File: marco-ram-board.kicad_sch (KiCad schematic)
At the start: 0 parts

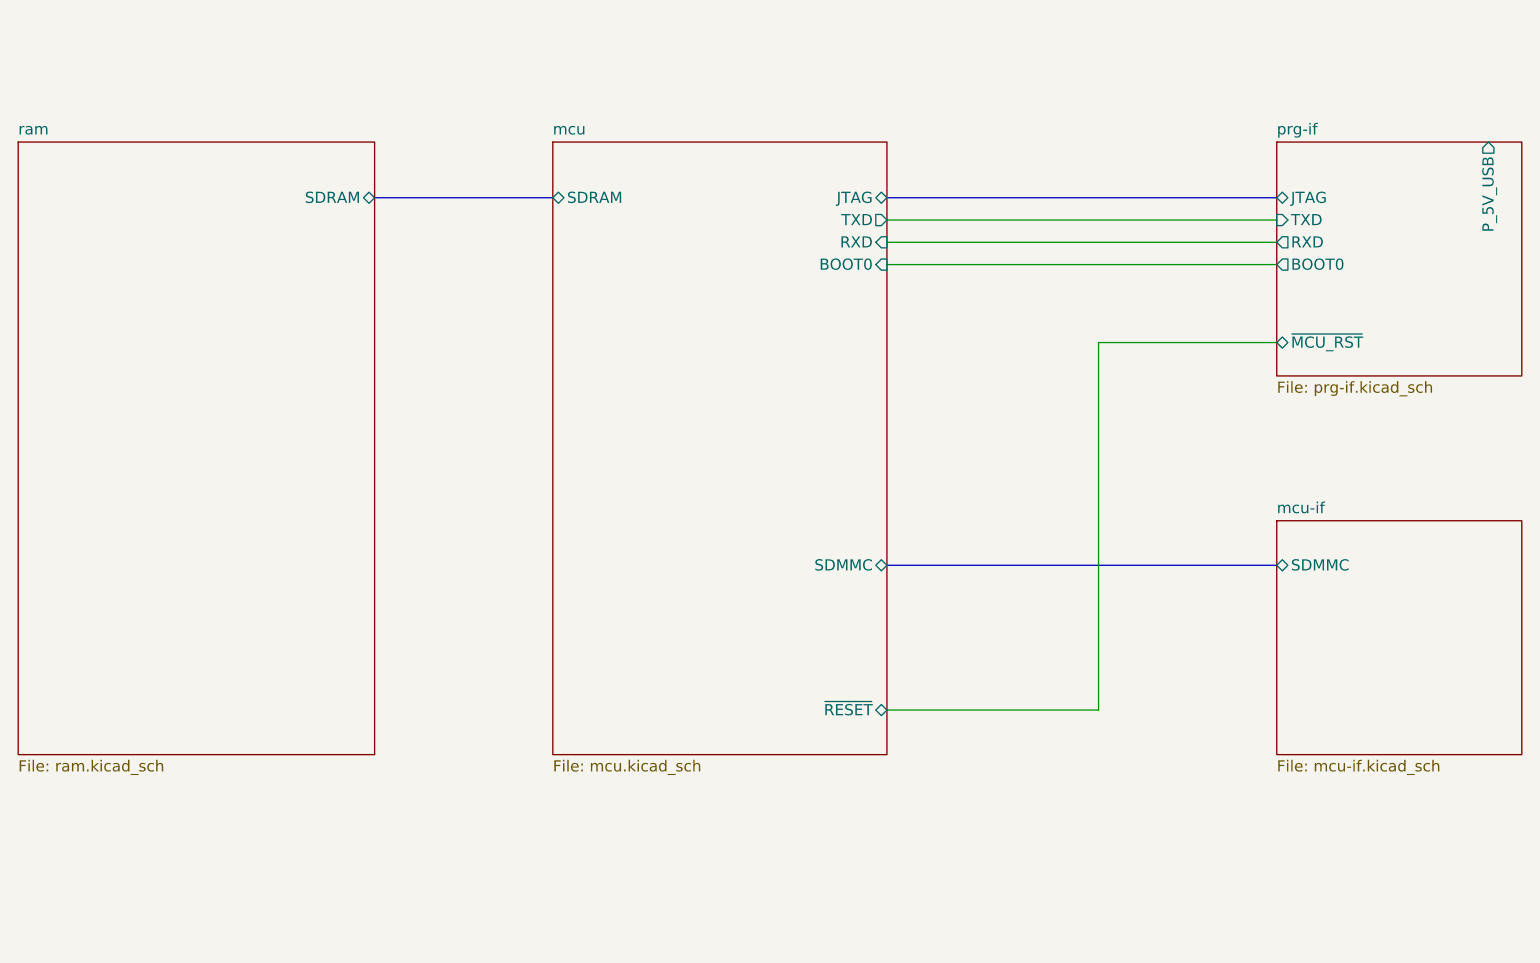
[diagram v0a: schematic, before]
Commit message: Add power supply.
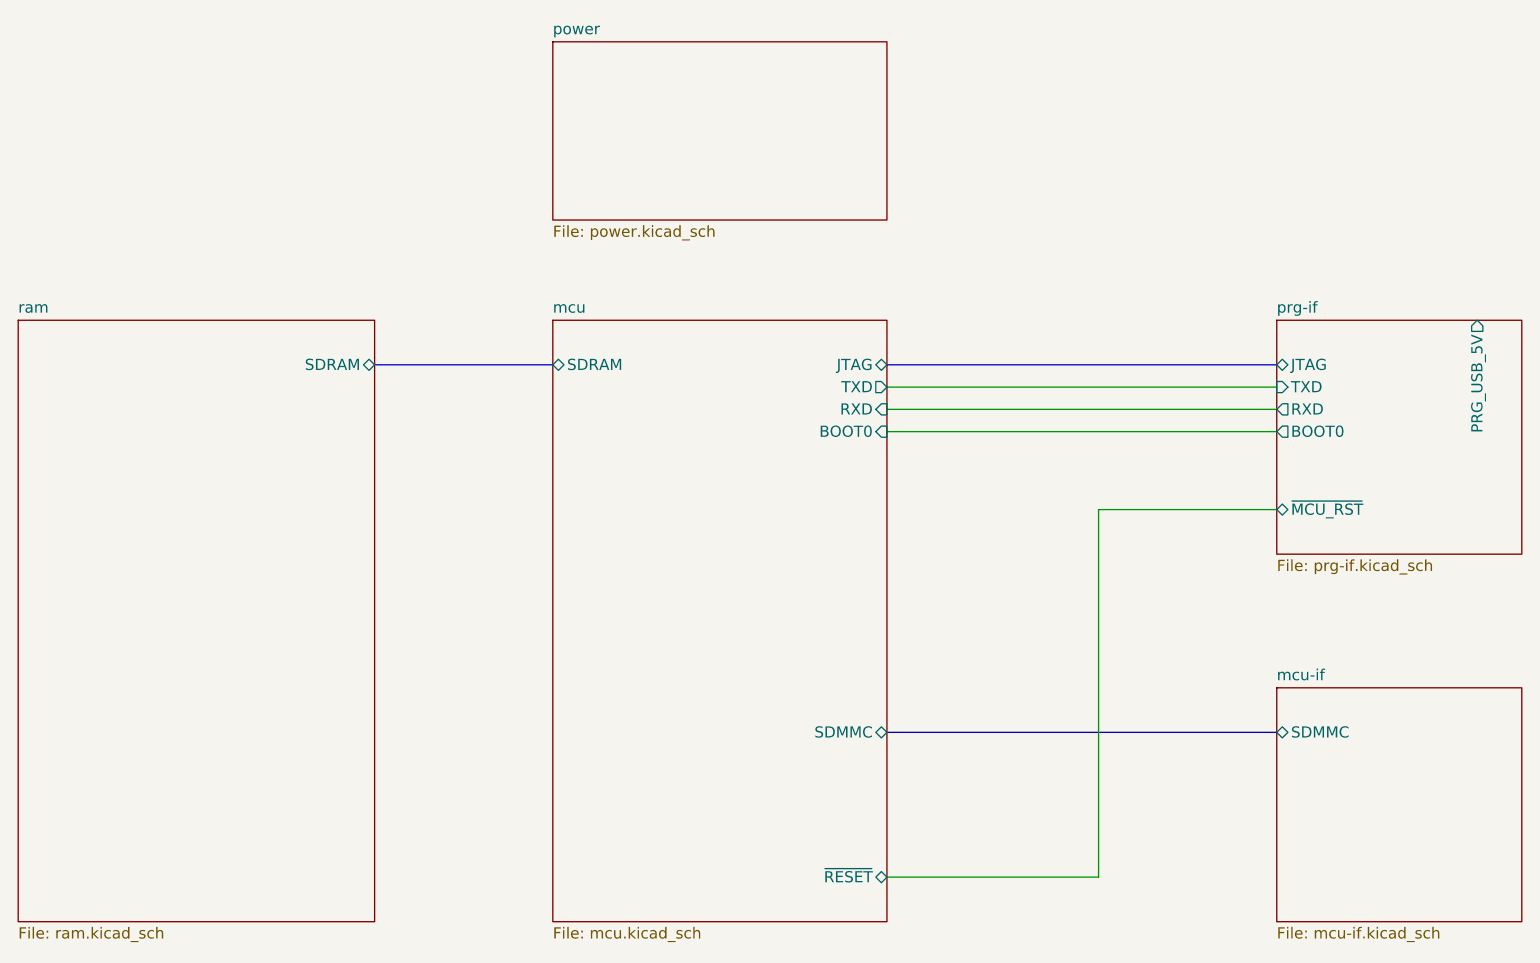
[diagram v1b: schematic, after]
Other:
- added sheet power (power.kicad_sch)
- sheet prg-if ports: added PRG_USB_5V; removed P_5V_USB
